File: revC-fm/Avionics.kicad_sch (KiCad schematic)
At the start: 76 parts, among them J1 5031821852, P2 TSM-105-01-F-SV, P3 FTSH-105-01-F-DV-K-TR, SW1 KMR231NG LFS, SW2 KMR231NG LFS, U4 imu-stamp-revA, U5 MAX708RESA-T, U6 SN74LVC1T45DCK, U7 MR25H40MDF, U8 ATSAMD51N20A-AUT, U9 DS1343D-33+, Y1 32.768kHz, Y2 32.768kHz

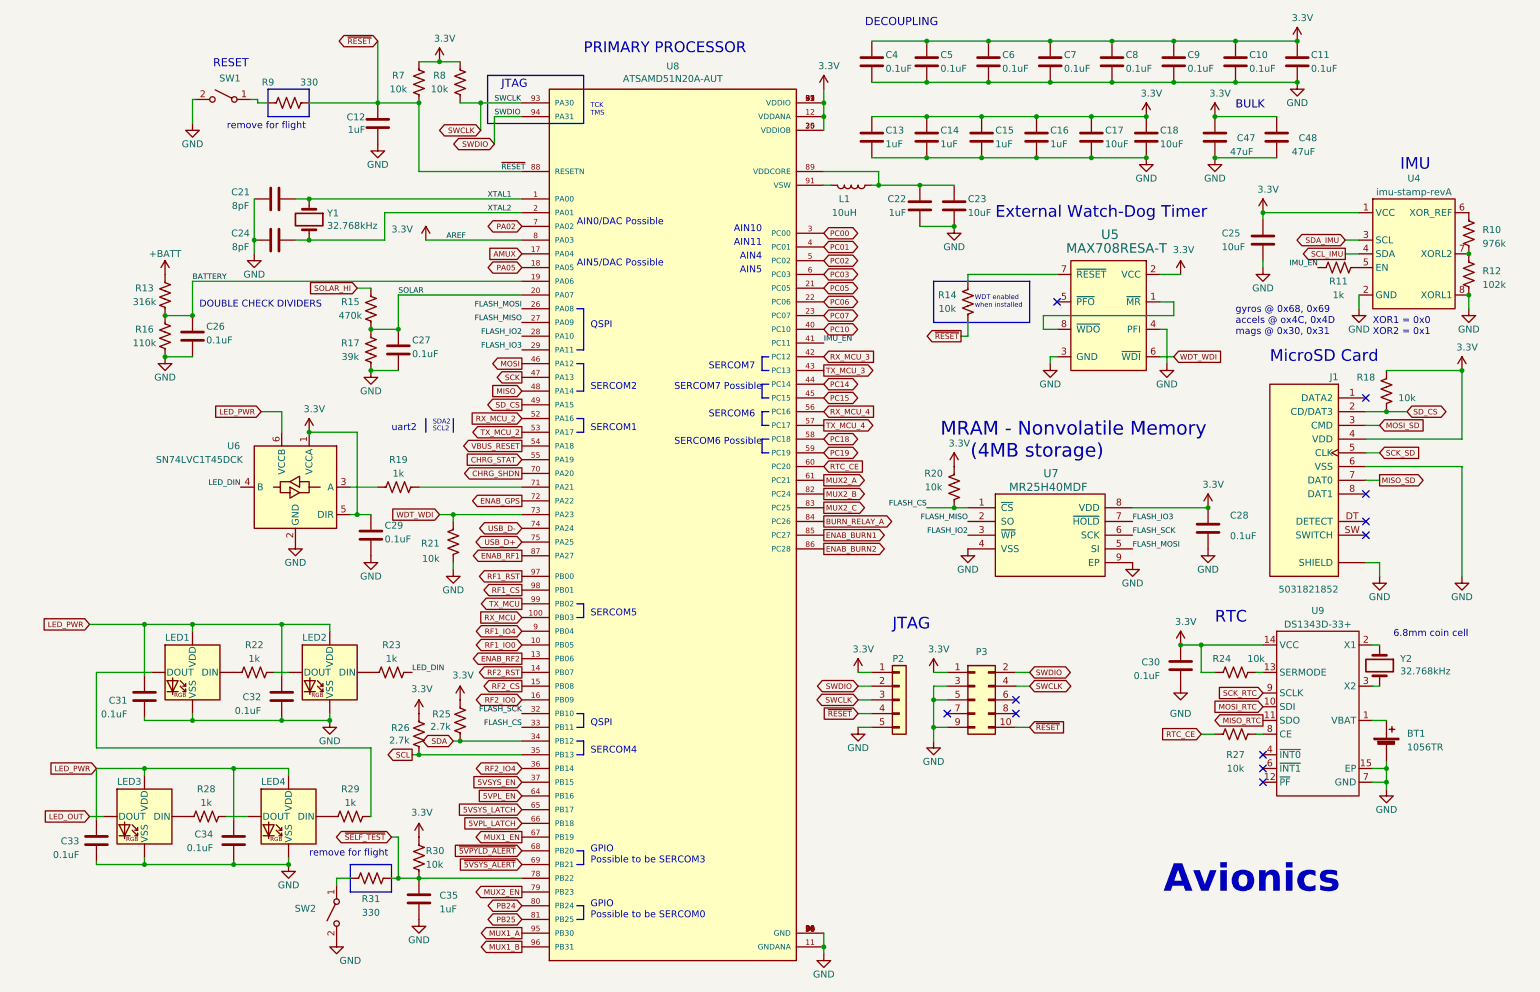
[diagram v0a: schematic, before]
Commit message: working revC
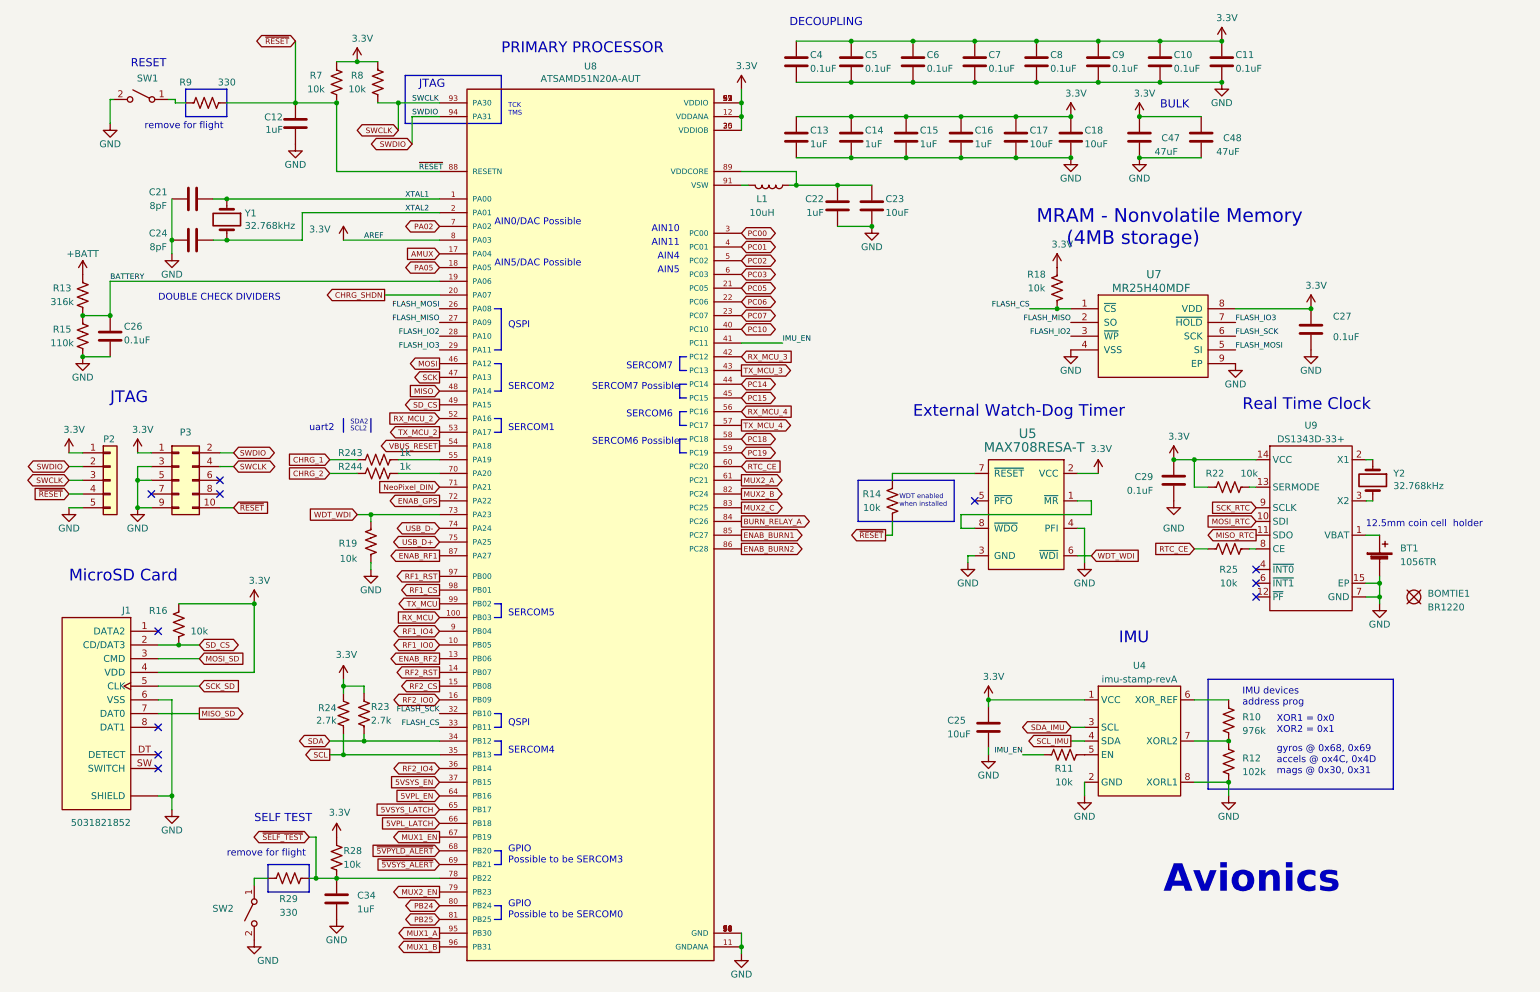
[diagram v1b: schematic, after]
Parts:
- removed C27, C29, C31, C32, C33, C34: 0.1uF, Capacitor_SMD:C_0603_1608Metric, symbol Device:C
- removed LED1, LED2, LED3, LED4: SK68xx-EC3210x, SierraLobo:LED_SK68xx-EC3210x, symbol SierraLobo:SK68xx-EC3210x
- removed R15: 470k, Resistor_SMD:R_0603_1608Metric, symbol Device:R_US
- removed R17: 39k, Resistor_SMD:R_0603_1608Metric, symbol Device:R_US
- removed R19, R22, R23, R28, R29: 1k, Resistor_SMD:R_0603_1608Metric, symbol Device:R_US
- removed U6: SN74LVC1T45DCK, Package_TO_SOT_SMD:SOT-363_SC-70-6, symbol Logic_LevelTranslator:SN74LVC1T45DCK
- added BOMTIE1: BR1220, symbol SierraLobo:BOMTIE
- added R243, R244: 1k, Resistor_SMD:R_0402_1005Metric, symbol Device:R_US
- C10, C11, C26, C4, C5, C6, C7, C8, C9: footprint Capacitor_SMD:C_0603_1608Metric -> Capacitor_SMD:C_0402_1005Metric
- C17, C18, C23, C25: Mfr. Part No (none) -> CGA4J1X7S1E106K125AE
- C27: renamed from C28; footprint Capacitor_SMD:C_0603_1608Metric -> Capacitor_SMD:C_0402_1005Metric
- C29: renamed from C30; footprint Capacitor_SMD:C_0603_1608Metric -> Capacitor_SMD:C_0402_1005Metric
- C47, C48: Mfr. Part No (none) -> C3216X5R1E476M160AC
- L1: Mfr. Part No (none) -> BCL322520RT-100M-D
- P2: Mfr. Part No (none) -> TSM-105-01-F-SV
- P3: Mfr. Part No (none) -> FTSH-105-01-F-DV-K-TR
- R11: value 1k -> 10k; footprint Resistor_SMD:R_0603_1608Metric -> Resistor_SMD:R_0402_1005Metric
- R14, R7, R8: footprint Resistor_SMD:R_0603_1608Metric -> Resistor_SMD:R_0402_1005Metric
- R16: renamed from R18; footprint Resistor_SMD:R_0603_1608Metric -> Resistor_SMD:R_0402_1005Metric
- R18: renamed from R20; footprint Resistor_SMD:R_0603_1608Metric -> Resistor_SMD:R_0402_1005Metric
- R19: renamed from R21; footprint Resistor_SMD:R_0603_1608Metric -> Resistor_SMD:R_0402_1005Metric
- R22: renamed from R24; footprint Resistor_SMD:R_0603_1608Metric -> Resistor_SMD:R_0402_1005Metric
- R25: renamed from R27; footprint Resistor_SMD:R_0603_1608Metric -> Resistor_SMD:R_0402_1005Metric
- R28: renamed from R30; footprint Resistor_SMD:R_0603_1608Metric -> Resistor_SMD:R_0402_1005Metric
- U5: Mfr. Part No (none) -> MAX708RESA-T
- U7: Mfr. Part No (none) -> MR25H40MDF
- U8: Mfr. Part No (none) -> ATSAMD51N20A-AUT
- U9: Mfr. Part No DS1344D-33+ -> DS1343D-33+
- Y1: Mfr. Part No (none) -> ABS07AIG-32.768KHZ-1-T
- renumbered C35 to C34, R16 to R15, R25 to R23, R26 to R24, R31 to R29
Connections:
- net SOLAR is gone; now on net CHRG_SHDN: U8.20 (PA07)
- net CHRG_SHDN: no longer U8.70 (PA20)
- net NeoPixel_DIN: now reaches U8.71 (PA21)
- net CHRG_STAT: no longer names the net of U8.55 (PA19)
- net CHRG_STAT: now also R243.1
- new net: R244.1, U8.70 (PA20)
- new net CHRG_1: R243.2
- new net CHRG_2: R244.2
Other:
- note added: "12.5mm coin cell holder"
- note added: "IMU devices address prog"
- note added: "Real Time Clock"
- note added: "SELF TEST"
- note removed: "6.8mm coin cell"
- note removed: "RTC"
- moved on the sheet: BT1, C10, C11, C12, C13, C14, C15, C16, C17, C18, C21, C22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
